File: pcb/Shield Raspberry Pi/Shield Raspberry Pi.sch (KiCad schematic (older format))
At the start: 54 parts, among them J1 Conn_01x03, J10 Conn_01x02, J2 Conn_01x03, J3 Conn_01x03, J4 Jack-DC, J5 Raspberry_Pi_2_3, J6 Conn_01x02, J7 Conn_01x02, J8 Conn_01x02, J9 Conn_01x02, K1 SANYOU RELAY, K2 SANYOU RELAY, Q1 2N7002, Q2 2N7002, Q3 2N7002, Q4 2N7002, Q5 2N7002, Q6 2N7002, Q7 2N7002, U1 MAX485E, U2 LM2596 5.0

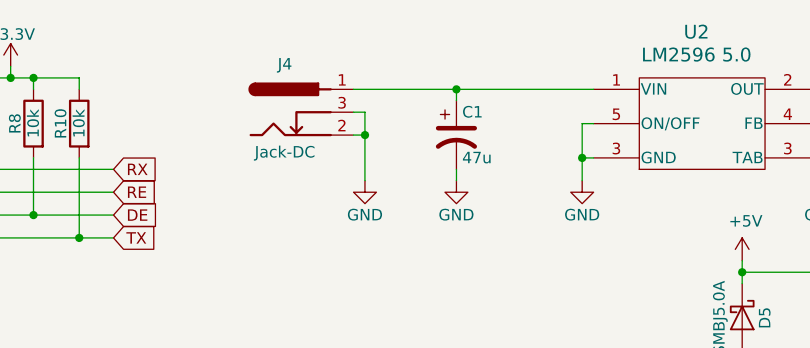
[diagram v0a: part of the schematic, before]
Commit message: Add files via upload
Version completamente ruteada, faltan solo algunas leyendas
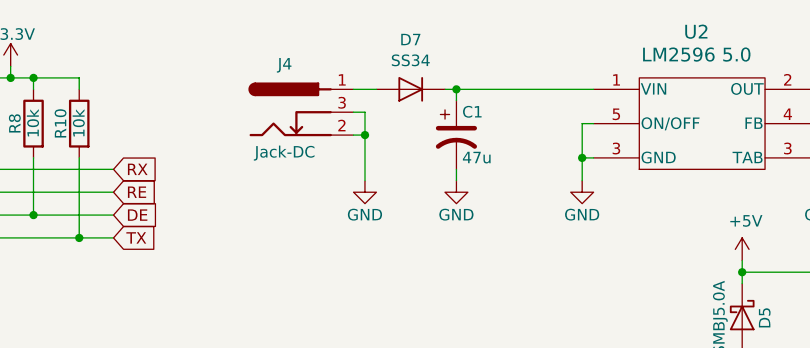
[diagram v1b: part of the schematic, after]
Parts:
- added D7: SS34, Diode_SMD:D_SMB, symbol Device:D
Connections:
- net at C1.1, U2.1 (VIN): now also D7.1 (K); no longer J4.1
- new net: D7.2 (A), J4.1
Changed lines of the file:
@@
 Wire Wire Line
 	4900 850  4900 800
-Wire Wire Line
-	4450 800  4900 800
 $Comp
 L Shield-Raspberry-Pi-rescue:GND-power #PWR017
@@
 	1    0    0    -1
 $EndComp
-Connection ~ 4900 800
 Wire Wire Line
 	4450 900  4500 900
@@
 Wire Wire Line
 	6150 1600 7000 1600
+$Comp
+L Device:D D7
+U 1 1 5DDA3987
+P 4700 800
+F 0 "D7" H 4700 584 50  0000 C CNN
+F 1 "SS34" H 4700 675 50  0000 C CNN
+F 2 "Diode_SMD:D_SMB" H 4700 800 50  0001 C CNN
+F 3 "~" H 4700 800 50  0001 C CNN
+	1    4700 800
+	-1   0    0    1
+$EndComp
+Wire Wire Line
+	4850 800  4900 800
+Connection ~ 4900 800
+Wire Wire Line
+	4550 800  4450 800
 $EndSCHEMATC
